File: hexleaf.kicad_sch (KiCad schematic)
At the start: 31 parts

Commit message: antenna parts
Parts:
- removed ANT?: 2450AT14A0100T, ANTC1608X40N, symbol hexleaf:2450AT14A0100T
- removed C? (x2): C_Small, symbol Device:C_Small
- removed L?: L_Small, symbol Device:L_Small
- added ANT1: AMCA31-2R450G-S1F-T3, hexleaf:ANTC3216X140N, symbol hexleaf:AMCA31-2R450G-S1F-T3
- added C8: 5p, Capacitor_SMD:C_0603_1608Metric, symbol Device:C_Small
- added L2: 1.8n, Inductor_SMD:L_0603_1608Metric, symbol Device:L_Small
- C6: renamed from C?; value C_Small -> 4p; footprint (none) -> Capacitor_SMD:C_0603_1608Metric; MFN (none) -> 81-GQM1875C2E4R0WB2D
- IC1: renamed from IC?; footprint QFN50P500X500X90-33N-D -> hexleaf:QFN50P500X500X90-33N-D
- J1: renamed from J?; footprint 009155004201006 -> hexleaf:009155004201006
- J2: renamed from J?; footprint (none) -> Connector_PinHeader_2.54mm:PinHeader_1x04_P2.54mm_Vertical
- L1: renamed from L?; value L_Small -> 2n; footprint (none) -> Capacitor_SMD:C_0402_1005Metric; MFN (none) -> 81-LQG15HZ2N0C02D
- PS1: renamed from PS?; footprint 009155004402006 -> hexleaf:009155004402006
- SW1, SW2: renamed from SW?; footprint (none) -> hexleaf:KXT3-1831561
- Y1: renamed from Y?; footprint ECS4001037B2CKMTR -> hexleaf:ECS4001037B2CKMTR
- gave numbers to parts that had none: 18
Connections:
- net ESP_EN: now also IC1.7 (CHIP_EN)
- net GND: now also C8.2
- net LNA_IN: now also C8.1, L2.2
- net at C6.1: now also ANT1.1 (FEED), L2.1
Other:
- note added: "50Ω Feed Line"
- note added: "Resources: https://www.espressif.com/sites/default/files/documentation/esp32-c3_hardware_design_guidelines_en.pdf Antenna: https://electronics.stackexchange.com/questions/598852/impedance-matching-for-esp32-d0wd-v3-qfn-5x5-connected-to-ufl-port https://www.eeweb.com/tools/pi-match/"
- note added: "TODO: - gpio setup (led, half-duplex uart) - edge-system and connections"
- note added: "π-network impedance matching esp: 35Ω + 10j, ant: 50Ω place close to RF output"
- note removed: "Resources: https://www.espressif.com/sites/default/files/documentation/esp32-c3_hardware_design_guidelines_en.pdf"
- note removed: "TODO: - antenna parts - button footprints - gpio setup (led, half-duplex uart) - edge-system and connections"
- moved on the sheet: C12, C6, IC1, R1

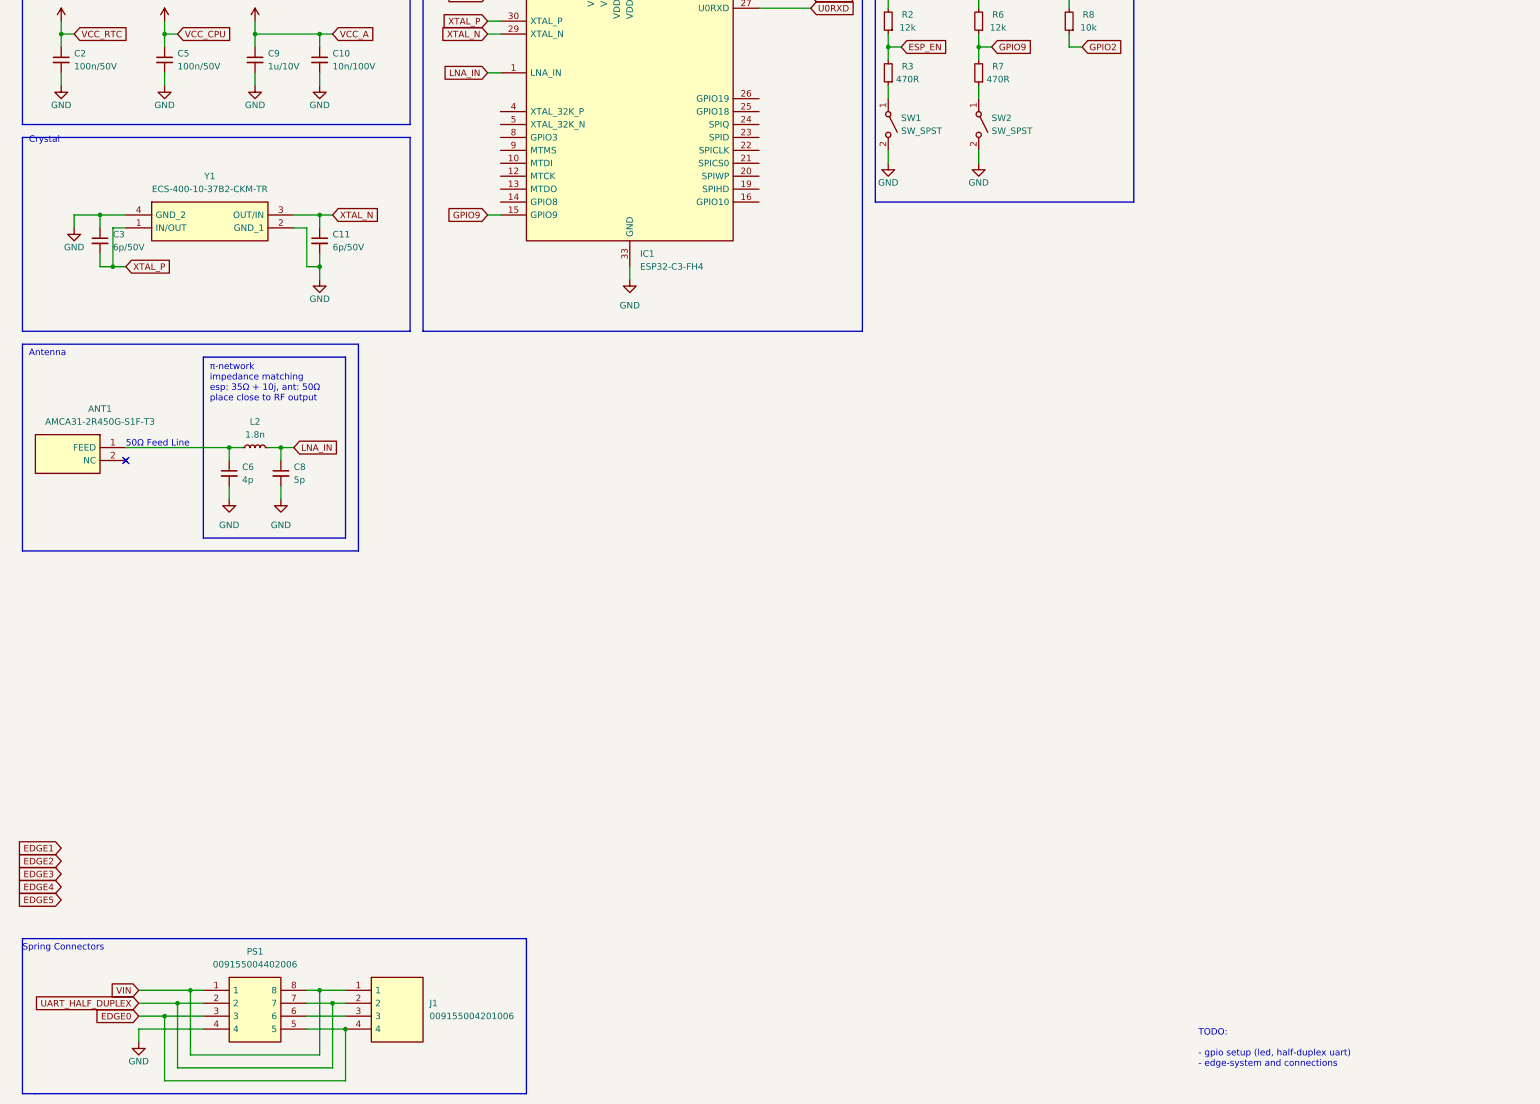
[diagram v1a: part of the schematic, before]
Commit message: updated todo
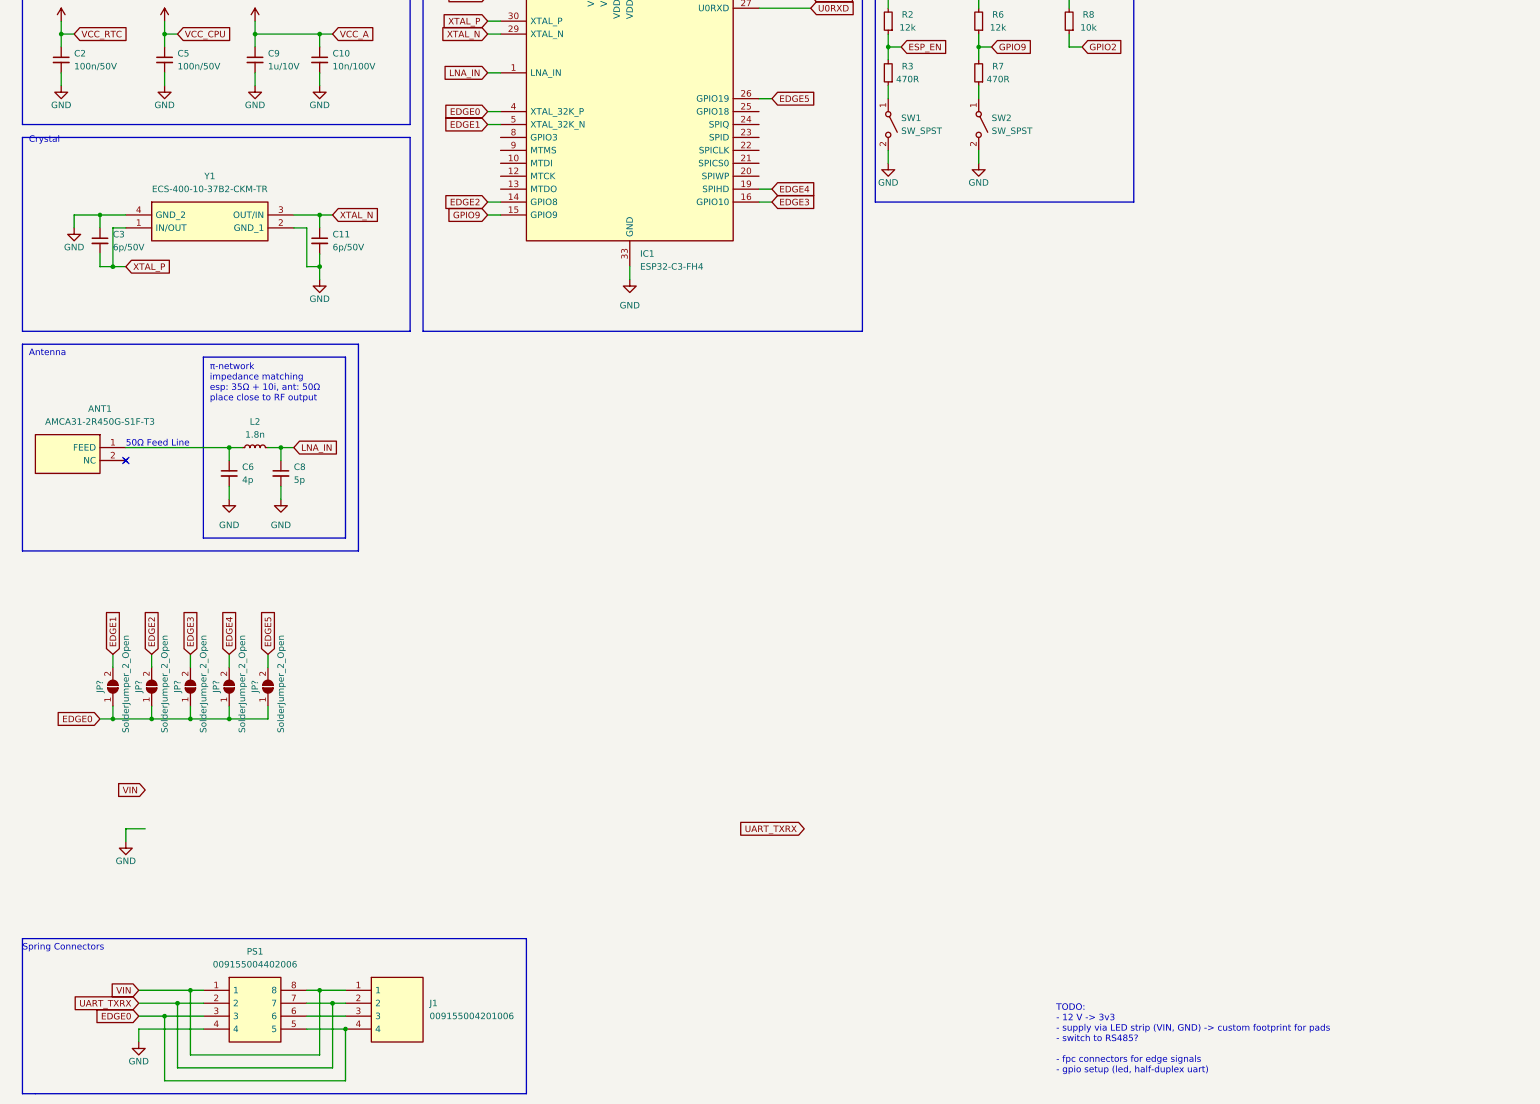
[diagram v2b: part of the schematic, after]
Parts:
- added JP? (x5): SolderJumper_2_Open, Jumper:SolderJumper-2_P1.3mm_Open_TrianglePad1.0x1.5mm, symbol Jumper:SolderJumper_2_Open
- IC1: Manufacturer_Part_Number ESP32-C3 -> ESP32-C3FH4; Mouser Part Number 356-ESP32-C3 -> 356-ESP32-C3FH4; Mouser Price/Stock https://www.mouser.co.uk/ProductDetail/Espressif-Systems/ES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 -> https://www.mouser.de/ProductDetail/Espressif-Systems/ESP32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
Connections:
- net EDGE0: now also IC1.4 (XTAL_32K_P), JP?.1 (A), JP?.1 (A), JP?.1 (A), JP?.1 (A), JP?.1 (A)
- net EDGE1: now also IC1.5 (XTAL_32K_N), JP?.2 (B)
- net EDGE2: now also IC1.14 (GPIO8), JP?.2 (B)
- net EDGE3: now also IC1.16 (GPIO10), JP?.2 (B)
- net EDGE4: now also IC1.19 (SPIHD), JP?.2 (B)
- net EDGE5: now also IC1.26 (GPIO19), JP?.2 (B)
- net UART_HALF_DUPLEX renamed UART_TXRX
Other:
- note added: "TODO: - 12 V -> 3v3 - supply via LED strip (VIN, GND) -> custom footprint for pads - switch to RS485? - fpc connectors for edge signals - gpio setup (led, half-duplex uart)"
- note added: "π-network impedance matching esp: 35Ω + 10i, ant: 50Ω place close to RF output"
- note removed: "TODO: - gpio setup (led, half-duplex uart) - edge-system and connections"
- note removed: "π-network impedance matching esp: 35Ω + 10j, ant: 50Ω place close to RF output"
